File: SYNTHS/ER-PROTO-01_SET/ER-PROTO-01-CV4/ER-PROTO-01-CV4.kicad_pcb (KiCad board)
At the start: 2 copper layers, 28 x 110 mm, 25 parts, among them J10 Conn_01x08, J11 Conn_01x10, J12 Conn_01x19, J13 Conn_01x19, J14 Conn_01x19, J15 Conn_01x19, J16 Conn_01x10, J17 Conn_01x10, J18 Conn_01x10, J19 Conn_01x10, J20 Conn_01x19, J21 Conn_01x10, J22 Conn_01x19, J37 PROTO01_POTS, J38 PROTO01_JACKS, J5 HEADER, 2X10, J6 HEADER, 2X8, J7 Conn_01x19, J8 Conn_01x19, J9 Conn_01x10, U1 MCP6004

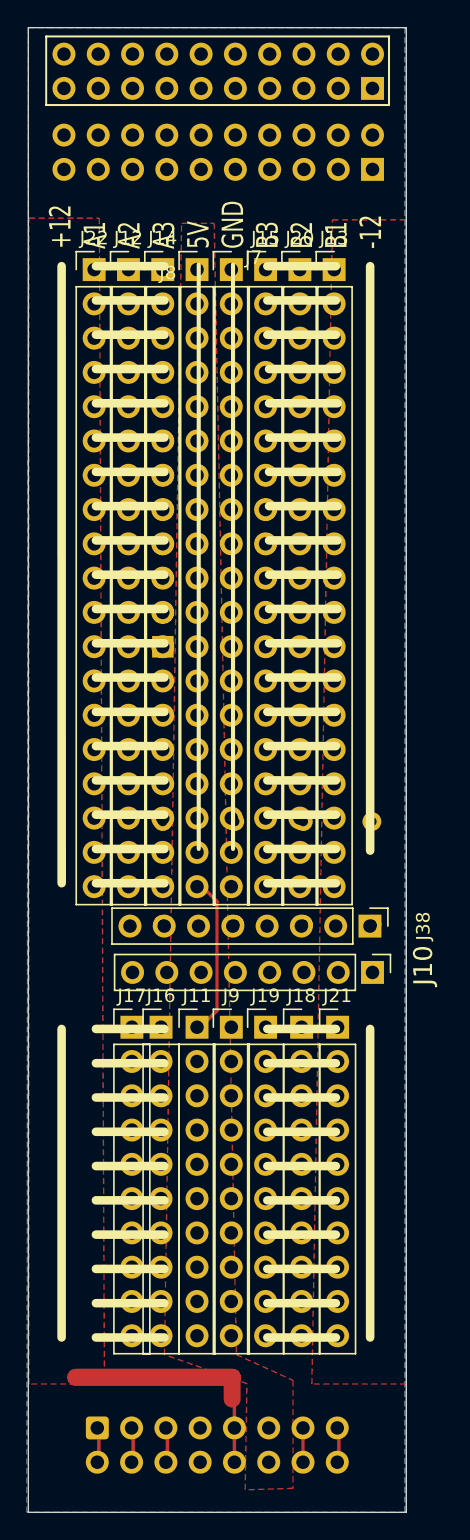
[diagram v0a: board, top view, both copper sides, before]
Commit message: pics
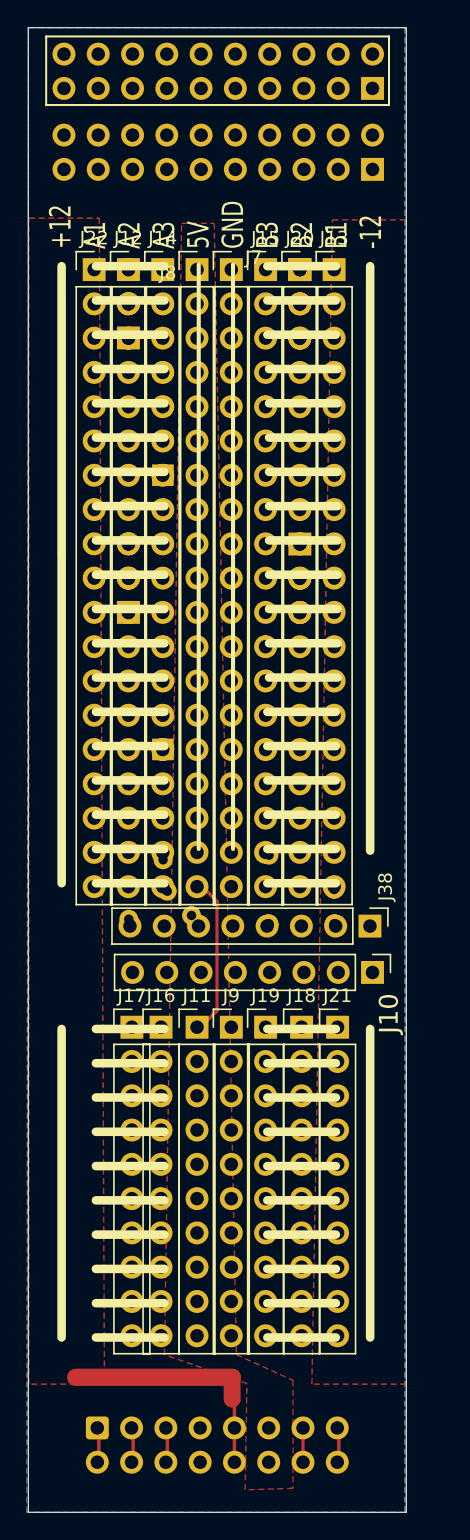
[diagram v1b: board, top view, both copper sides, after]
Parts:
- added H1: Conn_01x03, Connector_PinHeader_2.54mm:PinHeader_1x03_P2.54mm_Vertical, B.Cu at (105.9, 32.0)
- added H2: Conn_01x03, Connector_PinHeader_2.54mm:PinHeader_1x03_P2.54mm_Vertical, B.Cu at (118.6, 26.9)
- added H3: Conn_01x03, Connector_PinHeader_2.54mm:PinHeader_1x03_P2.54mm_Vertical, B.Cu at (105.9, 52.3)
- added H4: Conn_01x03, Connector_PinHeader_2.54mm:PinHeader_1x03_P2.54mm_Vertical, B.Cu at (118.6, 47.3)
- added U2: TL072, Package_DIP:DIP-8_W7.62mm, B.Cu at (108.5, 62.5)
- R5, R8: footprint Resistor_THT:R_Axial_DIN0204_L3.6mm_D1.6mm_P7.62mm_Horizontal -> Resistor_THT:R_Axial_DIN0204_L3.6mm_D1.6mm_P5.08mm_Vertical
- R6, R7: footprint Resistor_THT:R_Axial_DIN0204_L3.6mm_D1.6mm_P7.62mm_Horizontal -> Resistor_THT:R_Axial_DIN0204_L3.6mm_D1.6mm_P2.54mm_Vertical
- U1: value MCP6004 -> TL072; footprint Package_DIP:DIP-14_W7.62mm -> Package_DIP:DIP-8_W7.62mm
- moved R5 19.4 mm to (105.9, 75.1), turned to 60 degrees
- moved R7 14.8 mm to (121.2, 75.4), turned to 90 degrees
- moved U1 12.7 mm to (108.5, 42.2)
- moved R6 10.8 mm to (110.6, 74.8), turned to 135 degrees
- moved R8 7.98 mm to (116.3, 75.4), turned to 90 degrees
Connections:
- net /J1-S_X renamed /J4-S_X
- J37 pad 10: Net-(J37-Pad10) -> /VL1
- J37 pad 14: /L5V -> unconnected-(J37-Pad14)
- J37 pad 16: Net-(J37-Pad10) -> unconnected-(J37-Pad16)
- J37 pad 19: +5V -> unconnected-(J37-Pad19)
- J37 pad 5: unconnected-(J37-Pad5) -> /VH2
- J37 pad 7: GND -> /VL2
- J37 pad 8: /L5V -> /VH1
- J38 pad 1: /J1-T -> unconnected-(J38-Pad1)
- J38 pad 2: unconnected-(J38-Pad2) -> /J4-T
- J38 pad 3: /J3-T -> unconnected-(J38-Pad3)
- J38 pad 4: unconnected-(J38-Pad4) -> /J2-T
- J38 pad 5: /J2-T -> GND
- J38 pad 6: GND -> /J3-T
- J38 pad 7: /J4-T -> unconnected-(J38-Pad7)
- J38 pad 8: unconnected-(J38-Pad8) -> /J1-T
- J5 pad 10: /POT2-3 -> /POT1-3
- J5 pad 14: /POT1-1 -> /POT3-1
- J5 pad 16: /POT1-3 -> /POT3-3
- J5 pad 4: /POT2-3 -> unconnected-(J5-Pad4)
- J5 pad 5: /POT2-1 -> /POT3-1
- J5 pad 7: /POT2-3 -> /POT3-3
- J5 pad 8: /POT2-1 -> /POT1-1
- R5 pad 1: Net-(R5-Pad1) -> /J1-T
- R5 pad 2: /J1-T -> Net-(U1-Pad1)
- R6 pad 1: Net-(R6-Pad1) -> /J3-T
- R6 pad 2: /J3-T -> Net-(U2-Pad1)
- R7 pad 1: Net-(R7-Pad1) -> /J4-T
- R7 pad 2: /J4-T -> Net-(U2-Pad6)
- R8 pad 1: Net-(R8-Pad1) -> /J2-T
- R8 pad 2: /J2-T -> Net-(U1-Pad6)
- U1 pad 1: Net-(R6-Pad1) -> Net-(U1-Pad1)
- U1 pad 2: Net-(R6-Pad1) -> Net-(U1-Pad1)
- U1 pad 3: /POT3W -> /POT1W
- U1 pad 4: +5V -> /VL1
- U1 pad 5: /POT1W -> /POT2W
- U1 pad 6: Net-(R5-Pad1) -> Net-(U1-Pad6)
- U1 pad 7: Net-(R5-Pad1) -> Net-(U1-Pad6)
- U1 pad 8: Net-(R7-Pad1) -> /VH1
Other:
- board text added: "+12"
- board text added: "+5"
- board text added: "-12"
- board text added: "GND"
- board text removed: "RX TX RST GND D2 D5 D4 D5 D6 D7 D8 D9 D10 D11 D12"
- board text removed: "VIN GND RST +5V A7 A6 A5 A4 A3 A2 A1 A0 ARF 3V D13"
